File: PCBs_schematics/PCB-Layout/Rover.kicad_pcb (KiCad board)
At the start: 2 copper layers, 135 x 93 mm, 49 parts, among them J1 ToF-sensor2, J2 Pi-15,17, J3 Conn_01x02, J4 Conn_01x04, J5 Conn_01x04, J6 Conn_01x03, J7 USB-conn, M1 Sensor-DC-motor, M2 Wheel-dc-motor, M3 Motor_Servo, U1 TCST2103, U2 L293D, U3 ATMEGA168-20PU, U4 LLC_5V_3V3, U5 LM2576T-ADJ, U6 LM2576T-5, U7 INA219-breakout-board, Y1 Crystal

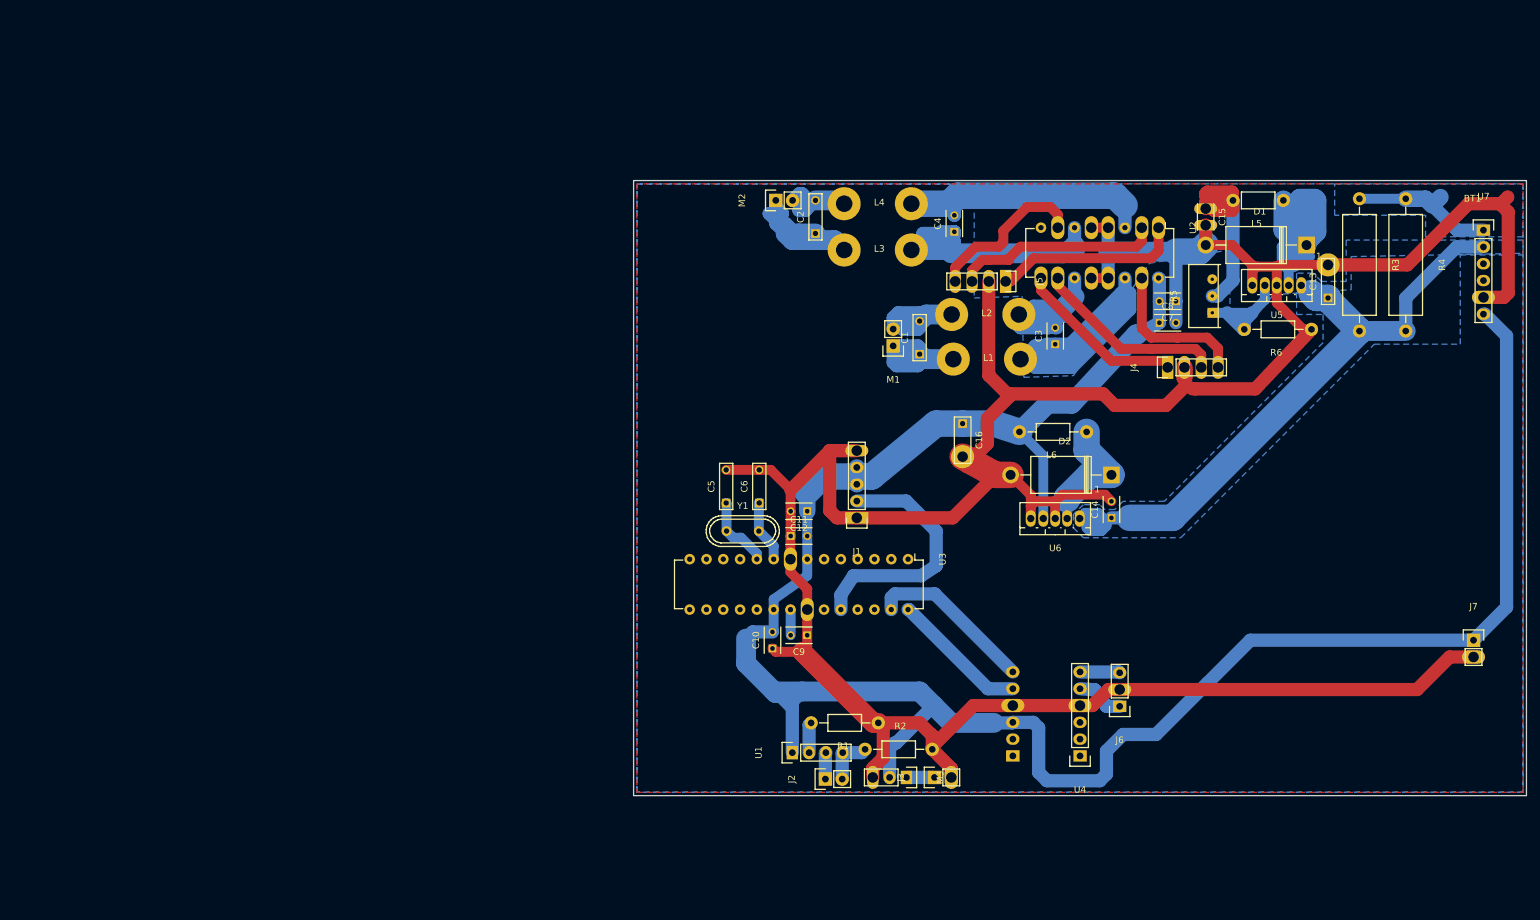
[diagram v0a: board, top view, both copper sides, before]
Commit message: more progress on the PCBs
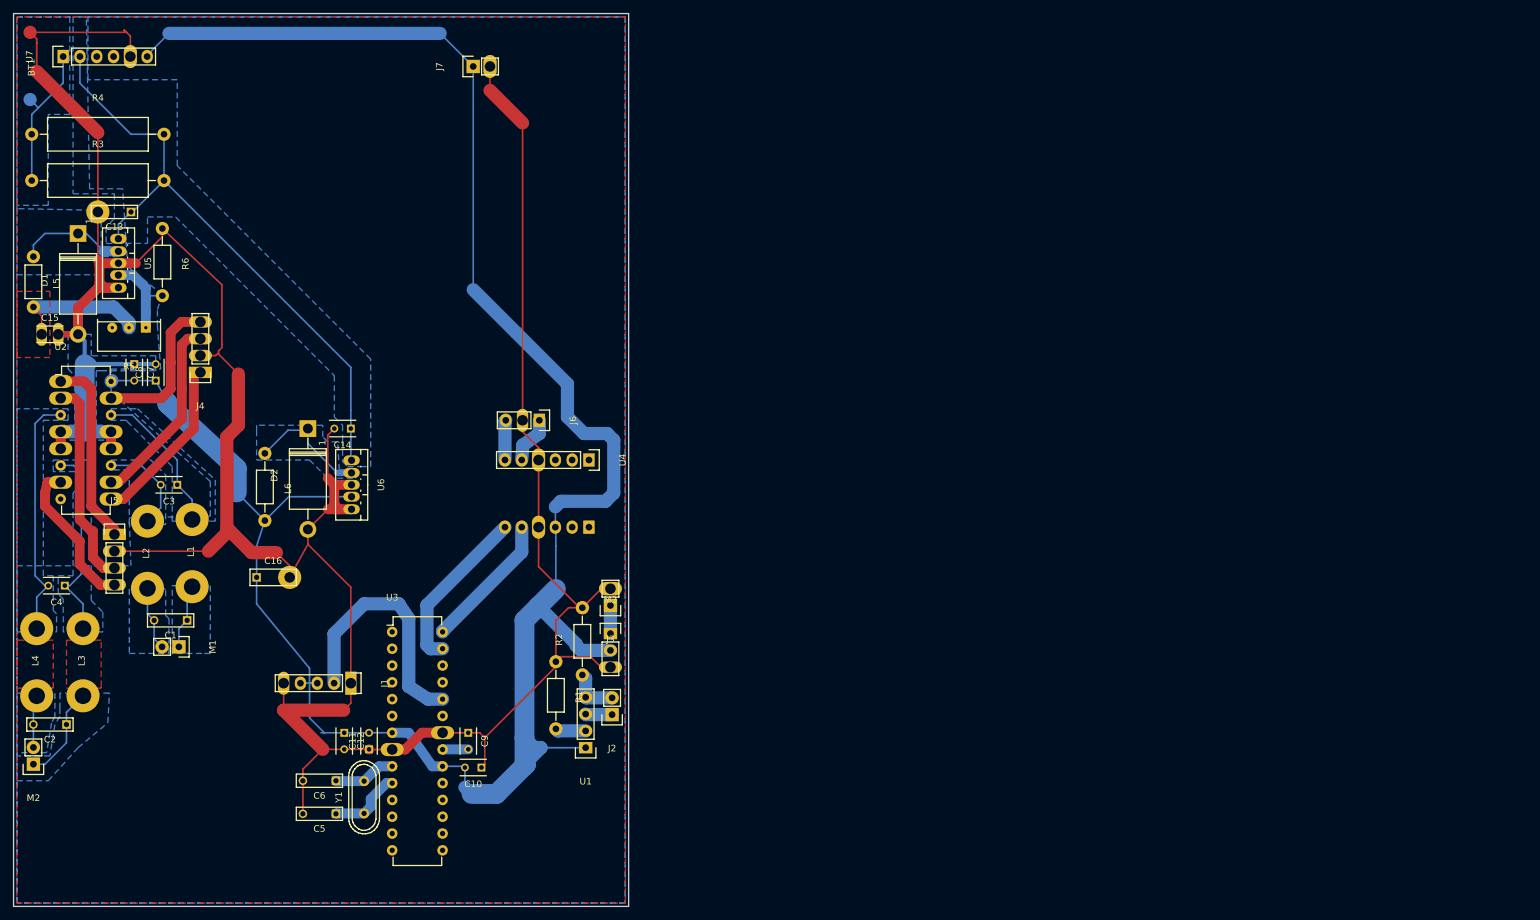
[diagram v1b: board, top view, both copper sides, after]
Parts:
- moved U7 216.3 mm to (31.2, 41.8), turned to 90 degrees
- moved BT1 213.8 mm to (26.2, 48.2), turned to 90 degrees
- moved R4 208.0 mm to (26.5, 53.5), turned to 0 degrees
- moved R3 200.8 mm to (26.5, 60.5), turned to 0 degrees
- moved L5 189.2 mm to (26.8, 72.0), turned to 270 degrees
- moved D1 185.8 mm to (33.5, 68.5), turned to 270 degrees
- moved C13 181.5 mm to (41.5, 65.2), turned to 180 degrees
- moved C15 177.0 mm to (28.0, 83.8), turned to 0 degrees
- moved U5 175.8 mm to (39.0, 73.0), turned to 270 degrees
- moved R6 174.4 mm to (46.2, 67.8), turned to 270 degrees
- moved J7 174.4 mm to (93.2, 43.2), turned to 90 degrees
- moved U2 167.6 mm to (30.9, 90.9), turned to 0 degrees
- moved R5 161.3 mm to (43.8, 82.8), turned to 180 degrees
- moved C7 157.8 mm to (42.0, 88.2), turned to 270 degrees
- moved C8 152.0 mm to (45.2, 90.8), turned to 90 degrees
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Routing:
- net Net-(C3-Pad1): track 73.9 -> 23.0 mm
- net Net-(D1-Pad1): track 46.9 -> 16.6 mm
- net Net-(C4-Pad1): track 44.8 -> 29.7 mm
- net Net-(C3-Pad2): track 28.6 -> 15.0 mm
- net Net-(C2-Pad1): track 26.9 -> 14.5 mm
- net +6V: track 33.3 -> 20.8 mm
- net Net-(C1-Pad1): track 21.8 -> 9.92 mm
- net Net-(C1-Pad2): track 20.6 -> 9.76 mm
- net +12V: track 102.2 -> 92.4 mm
- net Net-(C4-Pad2): track 42.6 -> 37.3 mm
- net Net-(C2-Pad2): track 12.7 -> 8.01 mm
- net GND: track 466.4 -> 470.7 mm
- net Net-(R5-Pad1): track 17.6 -> 13.8 mm
- net /Pi.27: track 24.9 -> 23.1 mm
- net Net-(D2-Pad1): track 20.0 -> 18.7 mm
- added copper zone on F.Cu, net (none)
- added copper zone on F.Cu, net +6V
- added copper zone on B.Cu, net GND
- added copper zone on B.Cu, net Net-(C1-Pad1)
- added copper zone on B.Cu, net Net-(C1-Pad2)
- added copper zone on B.Cu, net Net-(C2-Pad1)
- added copper zone on B.Cu, net Net-(C2-Pad2)
- added copper zone on B.Cu, net Net-(C3-Pad1)
- added copper zone on B.Cu, net Net-(C3-Pad2)
- added copper zone on B.Cu, net Net-(C4-Pad1)
- added copper zone on B.Cu, net Net-(C4-Pad2)
- added copper zone on B.Cu, net Net-(D1-Pad1)
- added copper zone on B.Cu, net Net-(D2-Pad1)
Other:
- board size 135 x 93 mm -> 93 x 135 mm
